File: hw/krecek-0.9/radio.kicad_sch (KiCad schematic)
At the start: 1 part, among them U12 CC1101RGPR

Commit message: Further tweaks and improvements
- Use a nicer schematic template
- Tie START button with power on
- Add ferrite to USB shield
- Add CC1/CC2 makeshift ADC
- Tidy up schematics a little bit

Signed-off-by: Jan Hamal Dvořák <mordae@anilinux.org>
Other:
- company: (none) -> DDM Spirála
- title: (none) -> Křeček
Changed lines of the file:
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@@
 (kicad_sch (version 20230121) (generator eeschema)
   (paper "A4")
+  (title_block
+    (title "Křeček")
+    (date "2023-12-20")
+    (rev "v0.9-wip")
+    (company "DDM Spirála")
+  )
   (hierarchical_label "RF_{MOSI}" (shape input) (at 121.92 105.41 180) (fields_autoplaced)
     (effects (font (size 1.27 1.27)) (justify right))

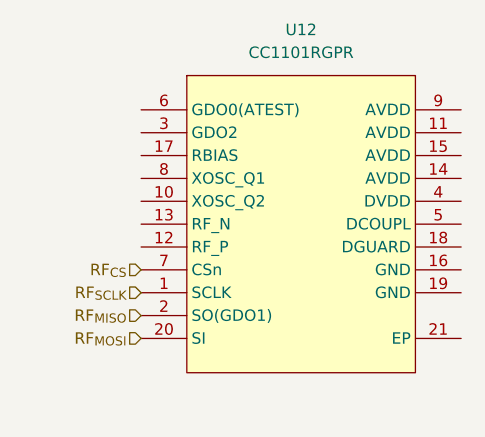
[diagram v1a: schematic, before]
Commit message: Complete most of the design, except for RF
Signed-off-by: Jan Hamal Dvořák <mordae@anilinux.org>
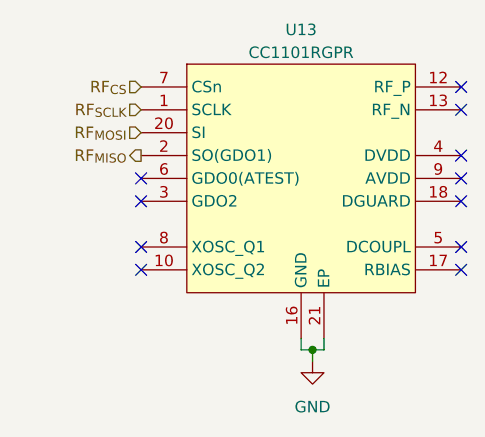
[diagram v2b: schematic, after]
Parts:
- renumbered U12 to U13
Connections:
- net AVDD: now reaches U13.11 (AVDD)
- net AVDD: now also U13.14 (AVDD), U13.15 (AVDD), U13.9 (AVDD)
- net GND: now reaches U13.16 (GND)
- net GND: now also U13.19 (GND), U13.21 (EP)
- no-connect marks 0 -> 11
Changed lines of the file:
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@@
     (company "DDM Spirála")
   )
-  (hierarchical_label "RF_{MOSI}" (shape input) (at 121.92 105.41 180) (fields_autoplaced)
+  (junction (at 140.97 106.68) (diameter 0) (color 0 0 0 0)
+  )
+  (no_connect (at 157.48 85.09))
+  (no_connect (at 157.48 80.01))
+  (no_connect (at 121.92 95.25))
+  (no_connect (at 157.48 97.79))
+  (no_connect (at 121.92 87.63))
+  (no_connect (at 157.48 95.25))
+  (no_connect (at 157.48 90.17))
+  (no_connect (at 121.92 97.79))
+  (no_connect (at 121.92 90.17))
+  (no_connect (at 157.48 77.47))
+  (no_connect (at 157.48 87.63))
+  (wire (pts (xy 140.97 106.68) (xy 139.7 106.68))
+    (stroke (width 0) (type default))
+  )
+  (wire (pts (xy 142.24 106.68) (xy 140.97 106.68))
+    (stroke (width 0) (type default))
+  )
+  (wire (pts (xy 140.97 106.68) (xy 140.97 107.95))
+    (stroke (width 0) (type default))
+  )
+  (wire (pts (xy 142.24 105.41) (xy 142.24 106.68))
+    (stroke (width 0) (type default))
+  )
+  (wire (pts (xy 139.7 106.68) (xy 139.7 105.41))
+    (stroke (width 0) (type default))
+  )
+  (hierarchical_label "RF_{MOSI}" (shape input) (at 121.92 82.55 180) (fields_autoplaced)
     (effects (font (size 1.27 1.27)) (justify right))
   )
-  (hierarchical_label "RF_{CS}" (shape input) (at 121.92 97.79 180) (fields_autoplaced)
+  (hierarchical_label "RF_{CS}" (shape input) (at 121.92 77.47 180) (fields_autoplaced)
     (effects (font (size 1.27 1.27)) (justify right))
   )
-  (hierarchical_label "RF_{SCLK}" (shape input) (at 121.92 100.33 180) (fields_autoplaced)
+  (hierarchical_label "RF_{SCLK}" (shape input) (at 121.92 80.01 180) (fields_autoplaced)
     (effects (font (size 1.27 1.27)) (justify right))
   )
-  (hierarchical_label "RF_{MISO}" (shape input) (at 121.92 102.87 180) (fields_autoplaced)
+  (hierarchical_label "RF_{MISO}" (shape output) (at 121.92 85.09 180) (fields_autoplaced)
     (effects (font (size 1.27 1.27)) (justify right))
+  )
+  (symbol (lib_id "power:GND") (at 140.97 107.95 0) (unit 1)
+    (in_bom yes) (on_board yes) (dnp no) (fields_autoplaced)
+    (property "Reference" "#PWR0106" (at 140.97 114.3 0)
+      (effects (font (size 1.27 1.27)) hide)
+    )
+    (property "Value" "GND" (at 140.97 113.03 0)
+      (effects (font (size 1.27 1.27)))
+    )
+    (property "Footprint" "" (at 140.97 107.95 0)
+      (effects (font (size 1.27 1.27)) hide)
+    )
+    (property "Datasheet" "" (at 140.97 107.95 0)
+      (effects (font (size 1.27 1.27)) hide)
+    )
+    (pin "1")
+    (instances
+      (project "krecek-0.9"
+        (path "/8888f37b-ecc2-47df-8824-4b4e1e726451/40971852-55ba-4d75-a9d8-2b5de9b08cbd"
+          (reference "#PWR0106") (unit 1)
+        )
+      )
+    )
   )
   (symbol (lib_id "LCSC:CC1101RGPR") (at 139.7 92.71 0) (unit 1)
     (in_bom yes) (on_board yes) (dnp no) (fields_autoplaced)
-    (property "Reference" "U12" (at 139.7 71.12 0)
+    (property "Reference" "U13" (at 139.7 71.12 0)
       (effects (font (size 1.27 1.27)))
     )
@@
       (project "krecek-0.9"
         (path "/8888f37b-ecc2-47df-8824-4b4e1e726451/40971852-55ba-4d75-a9d8-2b5de9b08cbd"
-          (reference "U12") (unit 1)
+          (reference "U13") (unit 1)
         )
       )
